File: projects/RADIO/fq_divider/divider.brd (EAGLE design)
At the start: 50 x 35 mm, 13 parts, among them IC1 SN74AC74D

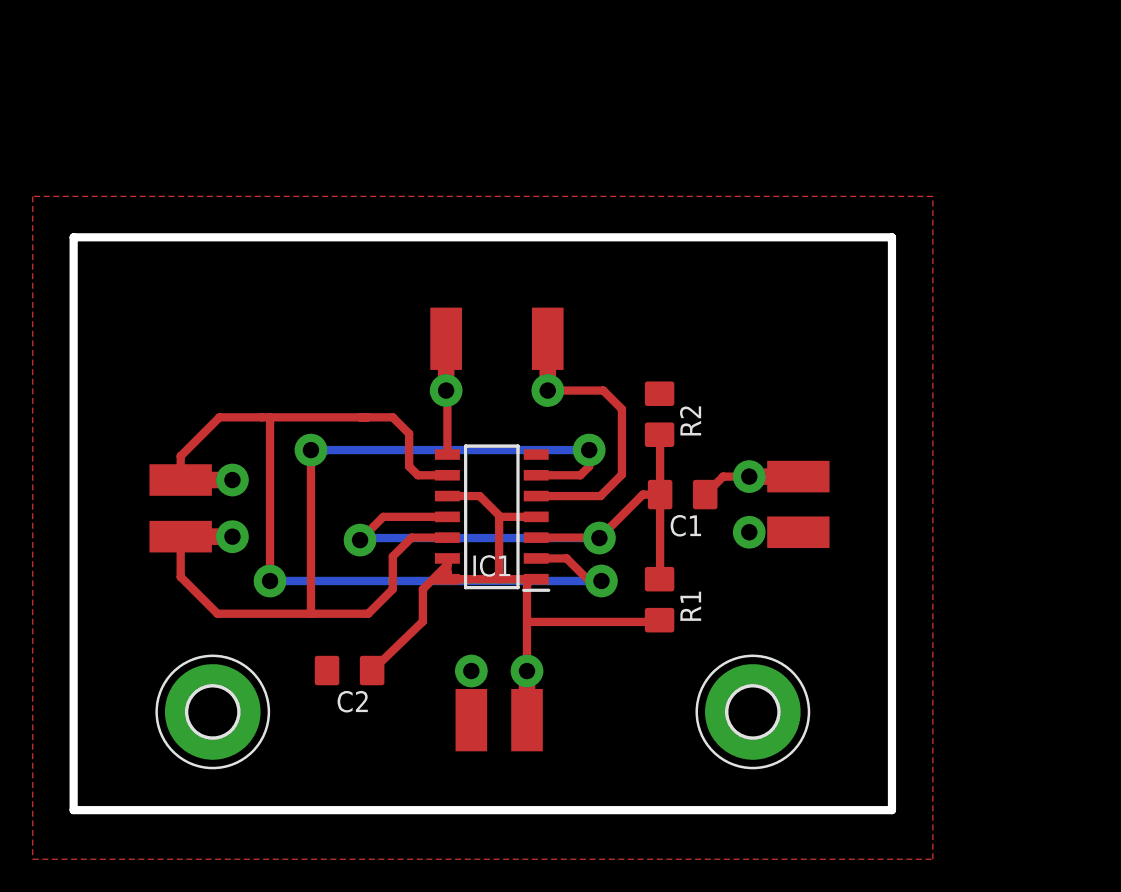
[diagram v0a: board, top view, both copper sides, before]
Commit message: update
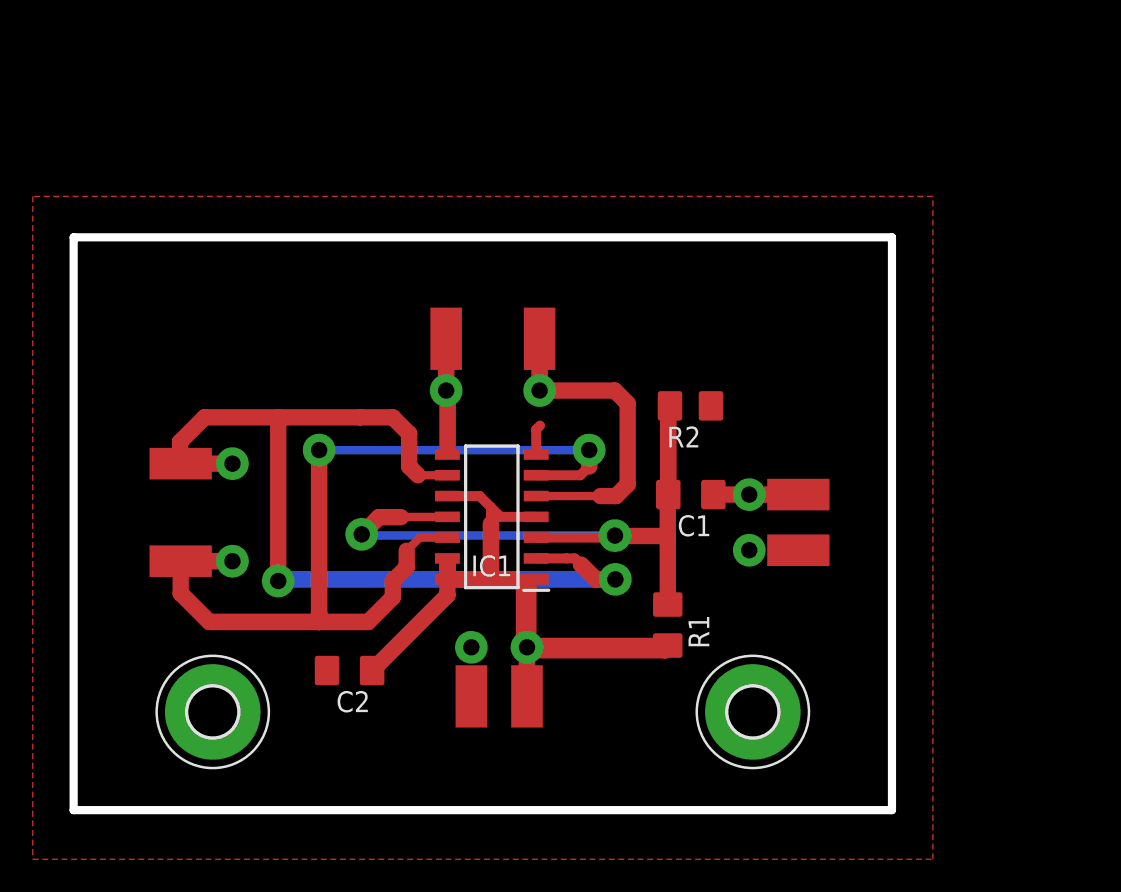
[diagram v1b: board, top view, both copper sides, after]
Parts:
- moved R2 1.96 mm to (37.7, 24.7), turned to 180 degrees
- moved R1 1.63 mm to (36.3, 11.3)
- moved RX_CLK0 1.50 mm to (6.54, 15.2)
- moved VCC 1.45 mm to (26.0, 6.95)
- moved LO_IN 1.10 mm to (44.3, 17.6)
- moved RX_CLK1 1.00 mm to (6.54, 21.2)
- moved C1 0.50 mm to (37.7, 19.3)
- moved TX_CLK0 0.50 mm to (28.5, 28.8)
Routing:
- net N$1: track 38.1 -> 41.2 mm
- net GND: track 0.00 -> 1.87 mm
- net QSE_CLK0: track 17.9 -> 19.7 mm
- net VCC: track 41.8 -> 43.2 mm
- net QSD_CLK1: track 59.9 -> 61.1 mm
- net N$2: track 6.15 -> 5.19 mm
- net QSD_CLK0: track 57.4 -> 56.9 mm

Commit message: Update
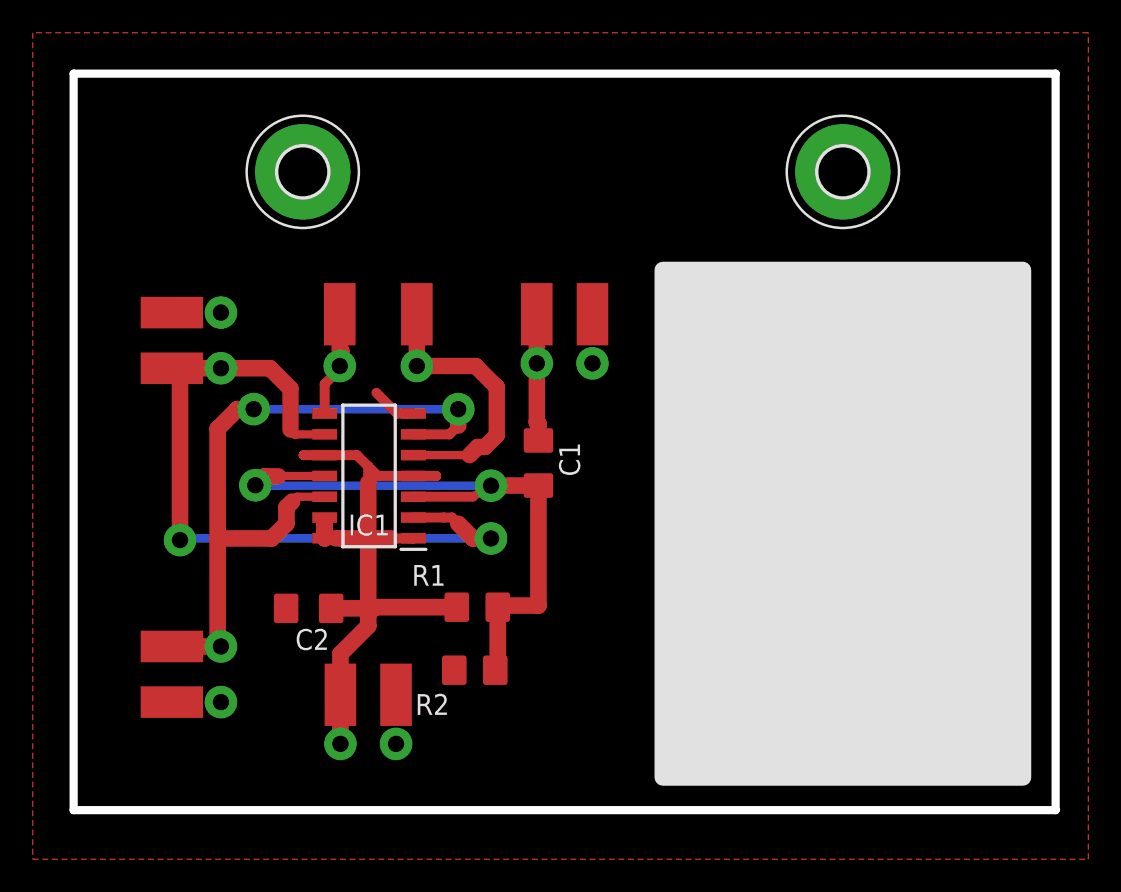
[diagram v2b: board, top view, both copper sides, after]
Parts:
- removed RX_CLK0, RX_CLK1: SMD_PTH_PIN, mylib:SMD_PTH_PIN
- added H3, H4: MOUNT-PAD-ROUND2.8, holes:2,8-PAD
- added QSD_CLK0, QSD_CLK1: 2X_SMD_PTH_PIN, mylib:2X_SMD_PTH
- moved H1 33.5 mm to (47.0, 39.0)
- moved H2 33.5 mm to (14.0, 39.0)
- moved R2 20.8 mm to (24.5, 8.55), turned to 0 degrees
- moved LO_IN 19.1 mm to (30.0, 30.3), turned to 270 degrees
- moved R1 11.7 mm to (24.7, 12.4), turned to 180 degrees
- moved C1 9.51 mm to (28.4, 21.2), turned to 270 degrees
- moved VCC 8.00 mm to (18.0, 7.05), turned to 270 degrees
- moved IC1 7.91 mm to (18.1, 20.4)
- moved TX_CLK0 7.65 mm to (21.0, 30.3)
- moved TX_CLK1 6.67 mm to (16.3, 30.3)
- moved C2 4.55 mm to (14.4, 12.3)
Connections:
- net GND: now also H3.B2,8, H4.B2,8, QSD_CLK0.P$2, QSD_CLK0.T$2, QSD_CLK1.P$1, QSD_CLK1.T$1
- net QSD_CLK0: now also QSD_CLK0.P$1, QSD_CLK0.T$1; no longer RX_CLK0.P$1, RX_CLK0.P$2
- net QSD_CLK1: now also QSD_CLK1.P$2, QSD_CLK1.T$2; no longer RX_CLK1.P$1, RX_CLK1.P$2
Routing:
- net QSD_CLK1: track 61.1 -> 46.8 mm
- net QSD_CLK0: track 56.9 -> 43.8 mm
- net QSE_CLK0: track 19.7 -> 17.1 mm
- net N$2: track 5.19 -> 7.75 mm
- net QSE_CLK1: track 7.11 -> 8.37 mm
- net GND: track 1.87 -> 2.79 mm
- net VCC: track 43.2 -> 44.1 mm
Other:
- board size 50 x 35 mm -> 60 x 45 mm
